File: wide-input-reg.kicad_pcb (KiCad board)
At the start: 2 copper layers, 92.7 x 67.6 mm, 80 parts, among them P1 MOLEX_43160-0102, P2 JST_GH_6_RA, P3 MOLEX_MINIFIT_JR_2x2_WAY, Q1 Si7852DP, Q2 Si7852DP, U1 INA219AID**, U2 LM5116

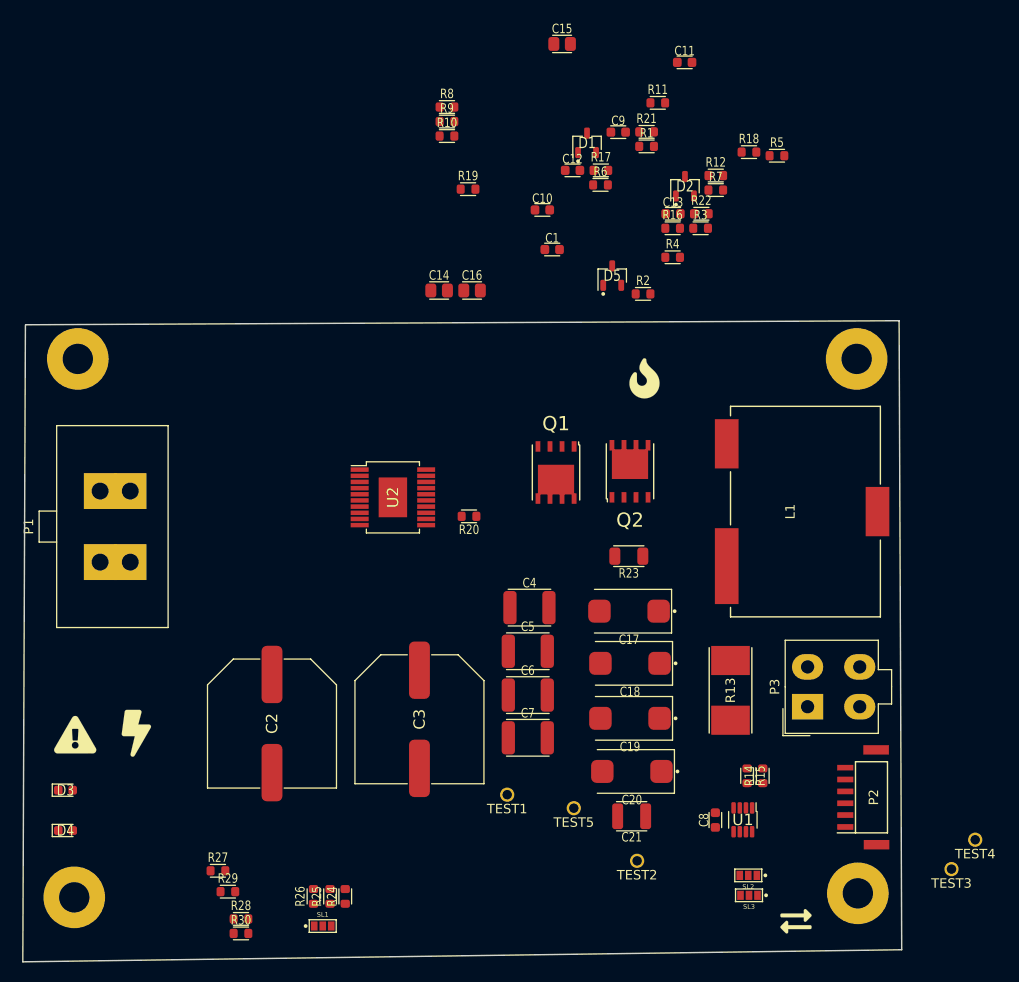
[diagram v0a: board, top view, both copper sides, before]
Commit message: Parts placement
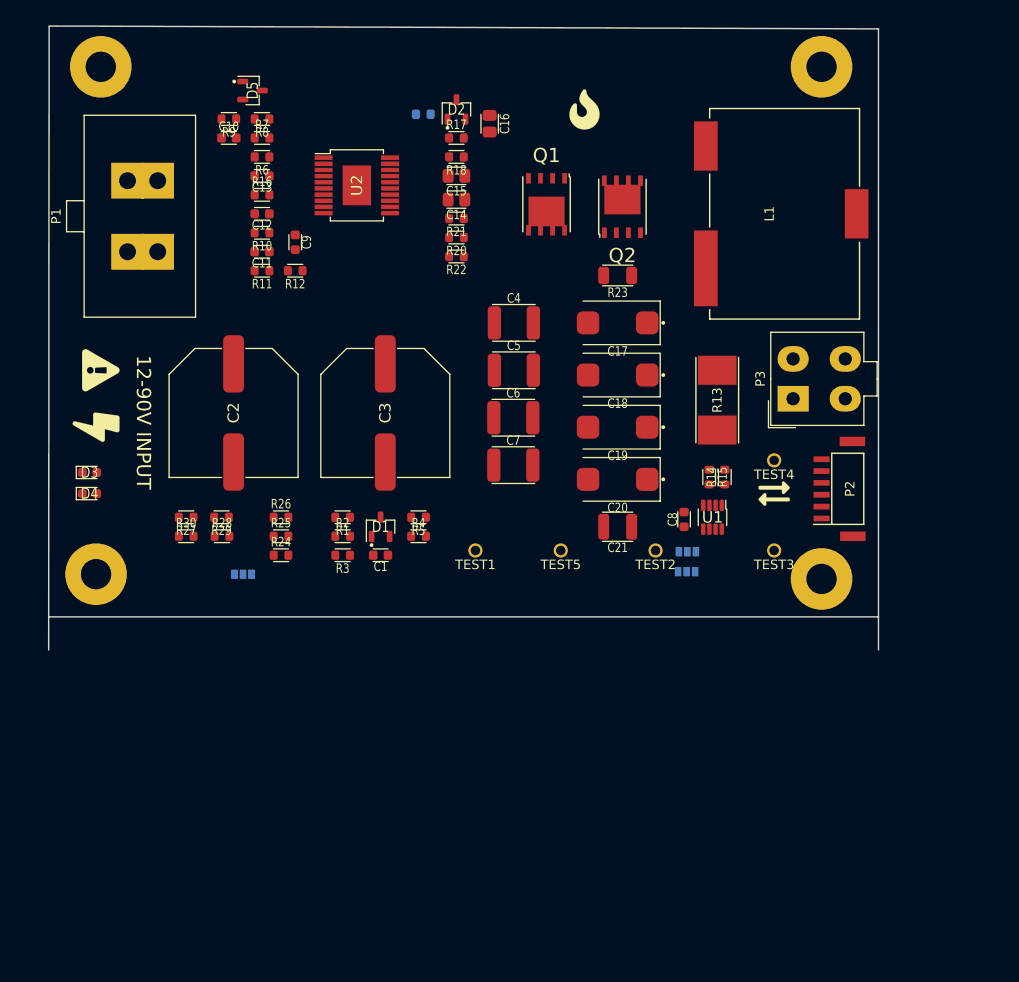
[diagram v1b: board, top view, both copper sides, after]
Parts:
- R19, SL1, SL2, SL3: moved to B.Cu
- moved R5 53.7 mm to (132.5, 120.0), turned to 180 degrees
- moved R3 51.1 mm to (124.5, 124.0), turned to 180 degrees
- moved R1 50.6 mm to (124.5, 120.0), turned to 180 degrees
- moved C11 48.8 mm to (116.0, 92.0), turned to 180 degrees
- moved R7 48.2 mm to (116.0, 80.0)
- moved D1 46.0 mm to (128.5, 121.0)
- moved R12 45.5 mm to (119.5, 94.0), turned to 180 degrees
- moved R11 45.3 mm to (116.0, 94.0), turned to 180 degrees
- moved TEST4 45.3 mm to (170.0, 114.0)
- moved LOGO4 45.2 mm to (170.0, 117.5), turned to 180 degrees
- moved C13 43.5 mm to (116.0, 84.0), turned to 180 degrees
- moved R16 43.4 mm to (116.0, 86.0)
- moved D5 42.7 mm to (115.0, 75.0), turned to 270 degrees
- moved R30 42.3 mm to (108.0, 122.0)
- moved R2 40.7 mm to (124.5, 122.0)
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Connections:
- R1 pad 2: +POWER -> +BATT
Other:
- board size 92.7 x 67.6 mm -> 87.5 x 65.8 mm
- board text added: "12-90V INPUT"
